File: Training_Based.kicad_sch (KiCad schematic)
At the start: 138 parts

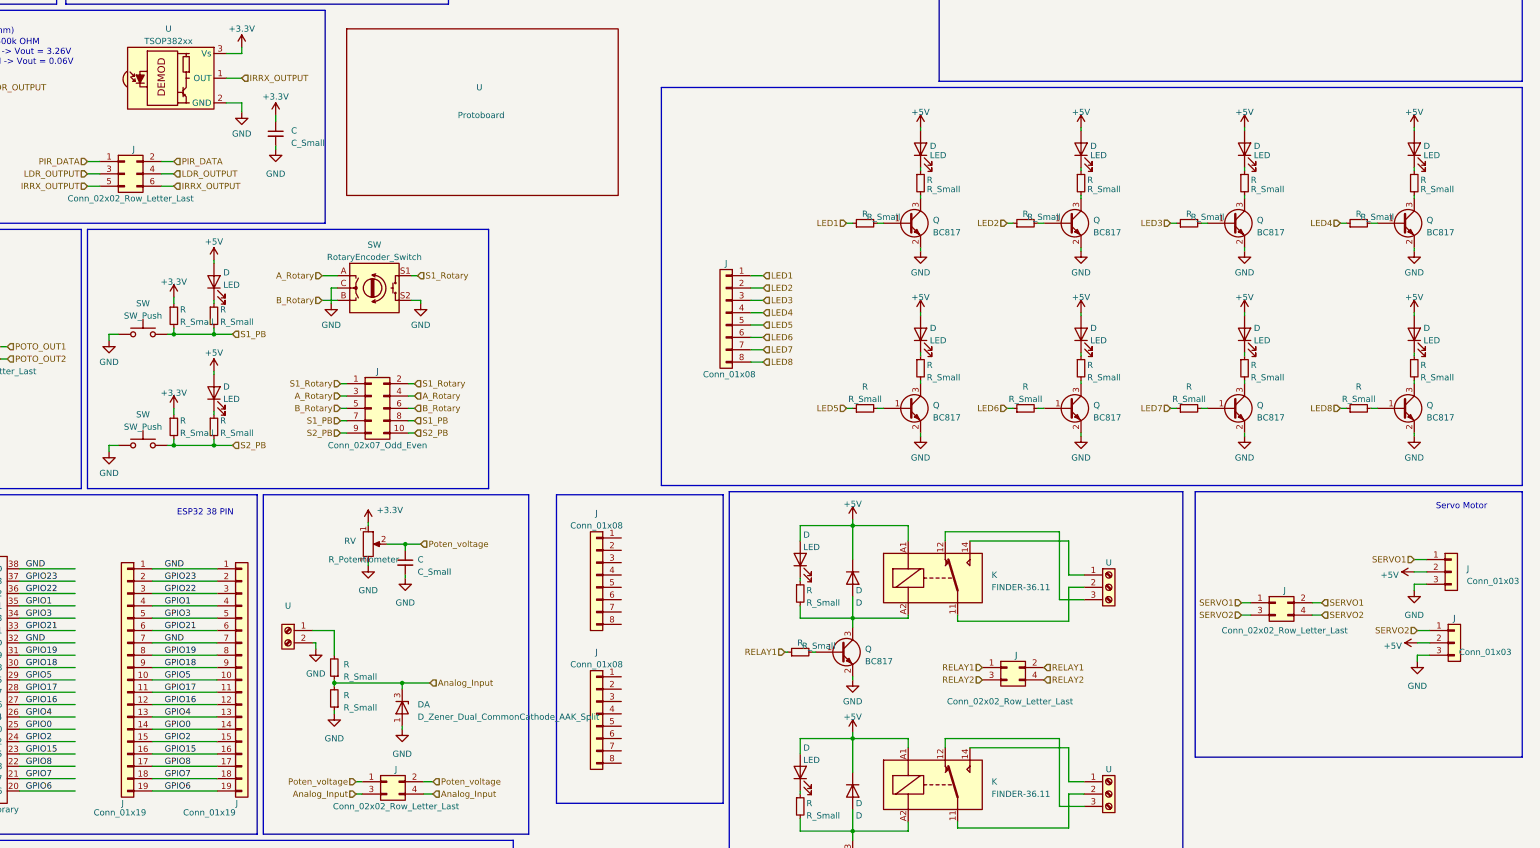
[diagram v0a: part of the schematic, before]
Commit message: Update Training_Based.kicad_sch
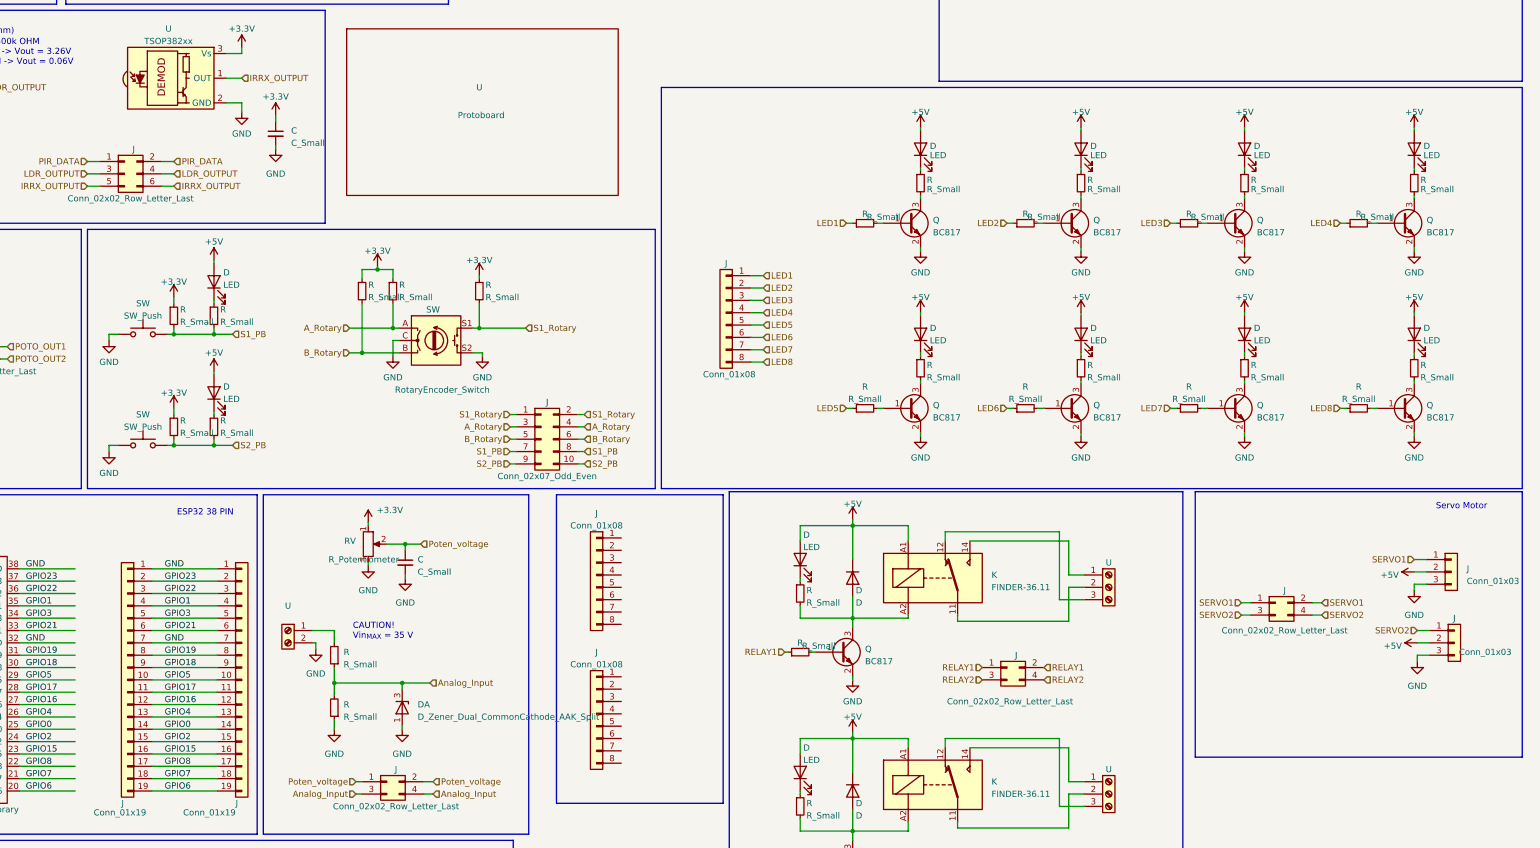
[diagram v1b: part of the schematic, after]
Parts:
- added R (x3): R_Small, symbol Device:R_Small
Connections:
- net +3.3V: now also R.1, R.1, R.1
- net A_Rotary: now also R.2
- net B_Rotary: now also R.2
- net S1_Rotary: now also R.2
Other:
- note added: "CAUTION! Vin_{MAX} = 35 V"
- moved on the sheet: J, R, SW
